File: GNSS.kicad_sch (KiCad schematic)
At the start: 0 parts

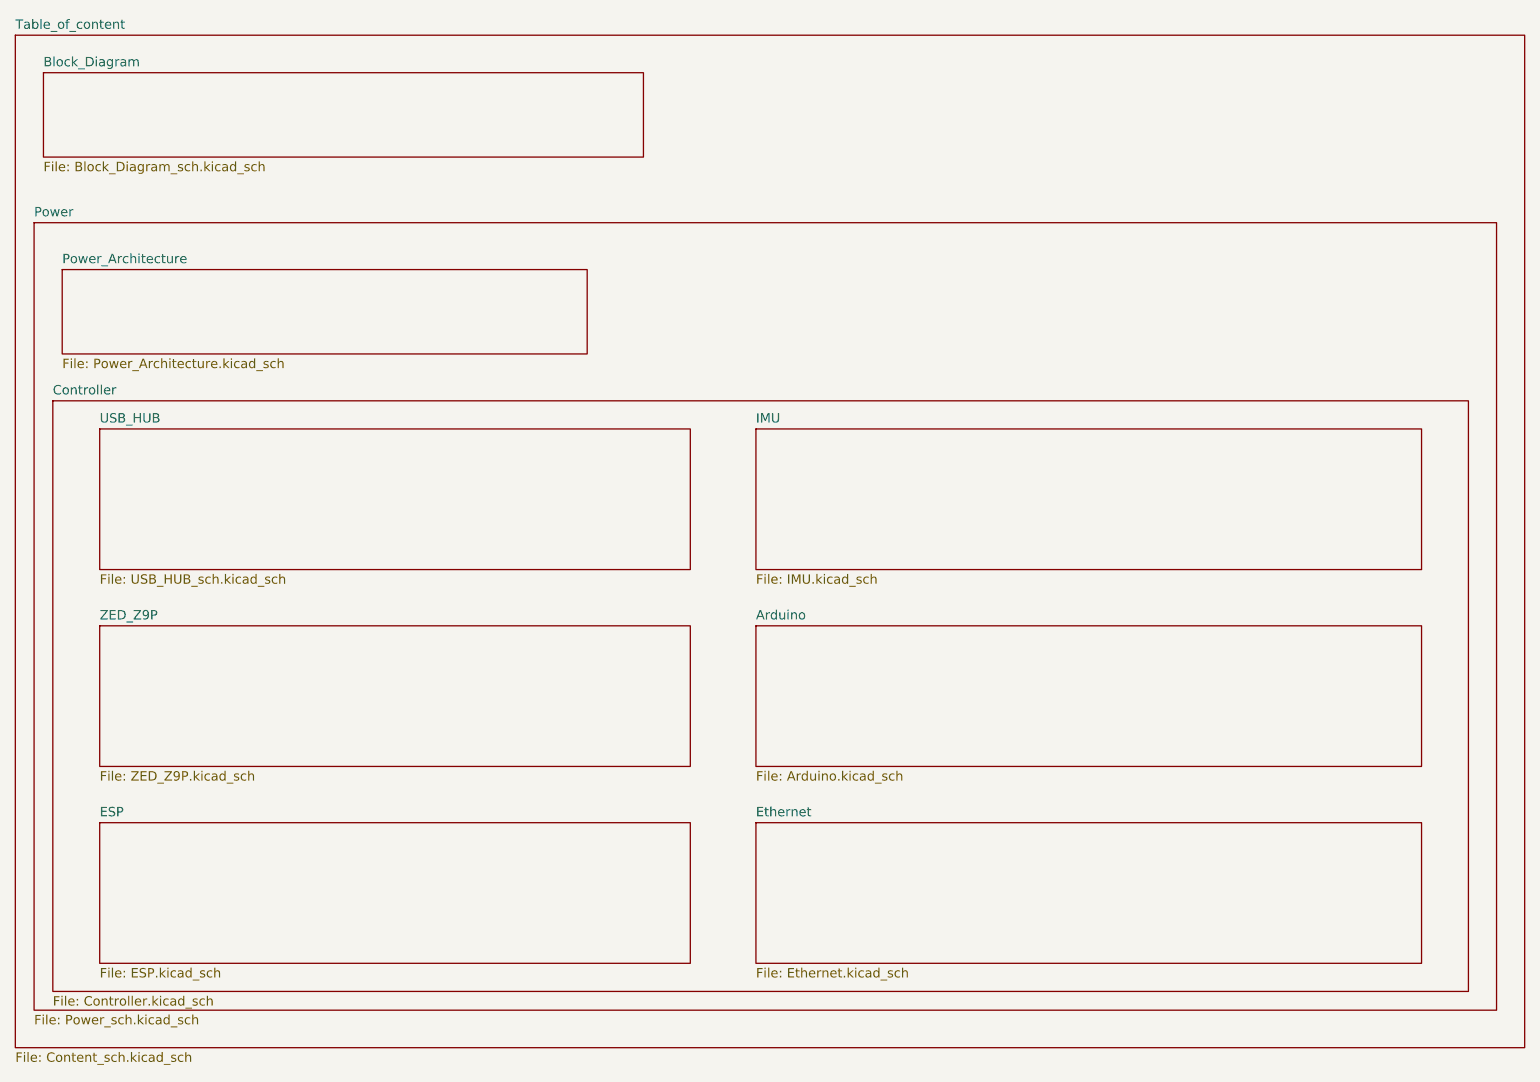
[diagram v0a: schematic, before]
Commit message: usb
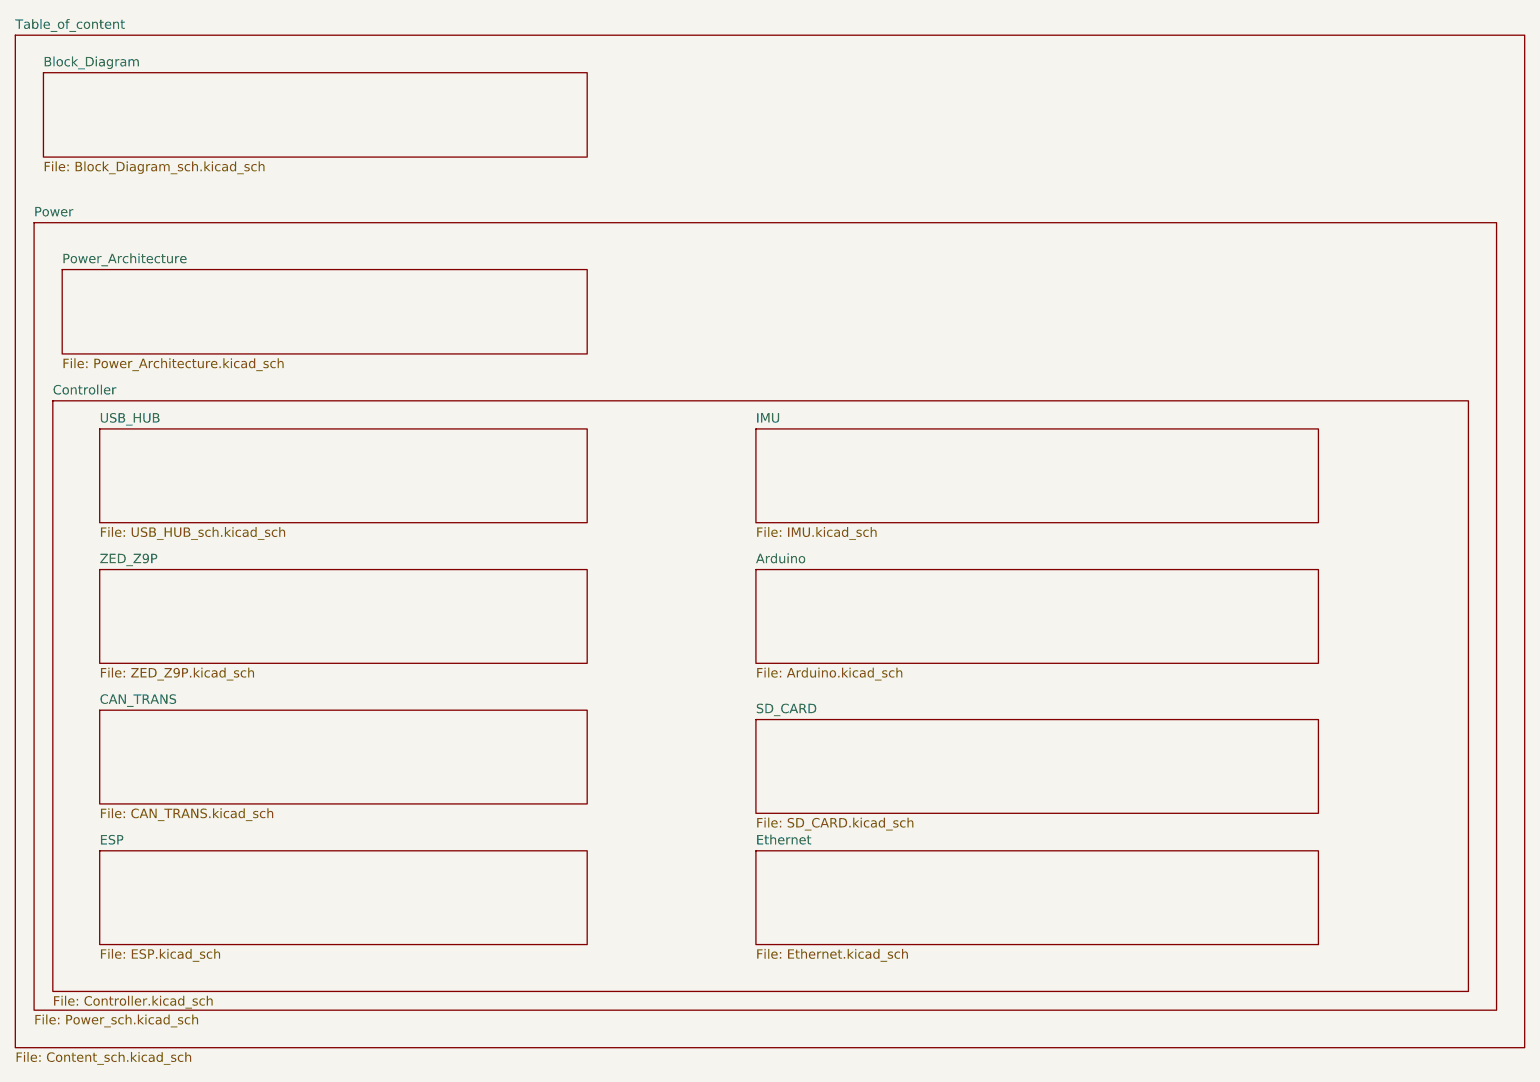
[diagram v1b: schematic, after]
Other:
- added sheet CAN_TRANS (CAN_TRANS.kicad_sch)
- added sheet SD_CARD (SD_CARD.kicad_sch)
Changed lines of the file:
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@@
 	(sheet
 		(at 137.16 74.93)
-		(size 90.17 19.05)
+		(size 76.2 12.7)
 		(fields_autoplaced yes)
 		(stroke
@@
 		)
 		(property "Sheetfile" "IMU.kicad_sch"
-			(at 137.16 94.5646 0)
+			(at 137.16 88.2146 0)
 			(effects
 				(font
@@
 	)
 	(sheet
-		(at 48.26 101.6)
-		(size 80.01 19.05)
+		(at 48.26 93.98)
+		(size 66.04 12.7)
 		(fields_autoplaced yes)
 		(stroke
@@
 		)
 		(property "Sheetname" "ZED_Z9P"
-			(at 48.26 100.8884 0)
+			(at 48.26 93.2684 0)
 			(effects
 				(font
@@
 		)
 		(property "Sheetfile" "ZED_Z9P.kicad_sch"
-			(at 48.26 121.2346 0)
+			(at 48.26 107.2646 0)
 			(effects
 				(font
@@
 	(sheet
 		(at 48.26 74.93)
-		(size 80.01 19.05)
+		(size 66.04 12.7)
 		(fields_autoplaced yes)
 		(stroke
@@
 		)
 		(property "Sheetfile" "USB_HUB_sch.kicad_sch"
-			(at 48.26 94.5646 0)
+			(at 48.26 88.2146 0)
 			(effects
 				(font
@@
 	(sheet
 		(at 40.64 26.67)
-		(size 81.28 11.43)
+		(size 73.66 11.43)
 		(fields_autoplaced yes)
 		(stroke
@@
 	)
 	(sheet
-		(at 137.16 128.27)
-		(size 90.17 19.05)
+		(at 137.16 132.08)
+		(size 76.2 12.7)
 		(fields_autoplaced yes)
 		(stroke
@@
 		)
 		(property "Sheetname" "Ethernet"
-			(at 137.16 127.5584 0)
+			(at 137.16 131.3684 0)
 			(effects
 				(font
@@
 		)
 		(property "Sheetfile" "Ethernet.kicad_sch"
-			(at 137.16 147.9046 0)
+			(at 137.16 145.3646 0)
 			(effects
 				(font
@@
 	)
 	(sheet
-		(at 137.16 101.6)
-		(size 90.17 19.05)
+		(at 137.16 93.98)
+		(size 76.2 12.7)
 		(fields_autoplaced yes)
 		(stroke
@@
 		)
 		(property "Sheetname" "Arduino"
-			(at 137.16 100.8884 0)
+			(at 137.16 93.2684 0)
 			(effects
 				(font
@@
 		)
 		(property "Sheetfile" "Arduino.kicad_sch"
-			(at 137.16 121.2346 0)
+			(at 137.16 107.2646 0)
 			(effects
 				(font
@@
 	)
 	(sheet
-		(at 48.26 128.27)
-		(size 80.01 19.05)
+		(at 137.16 114.3)
+		(size 76.2 12.7)
+		(fields_autoplaced yes)
+		(stroke
+			(width 0.1524)
+			(type solid)
+		)
+		(fill
+			(color 0 0 0 0.0000)
+		)
+		(property "Sheetname" "SD_CARD"
+			(at 137.16 113.5884 0)
+			(effects
+				(font
+					(size 1.27 1.27)
+				)
+				(justify left bottom)
+			)
+		)
+		(property "Sheetfile" "SD_CARD.kicad_sch"
+			(at 137.16 127.5846 0)
+			(effects
+				(font
+					(size 1.27 1.27)
+				)
+				(justify left top)
+			)
+		)
+		(instances
+			(project "GNSS"
+				(path "/a70dad34-b24c-4b58-b91c-f14576b5da7d"
+					(page "14")
+				)
+			)
+		)
+	)
+	(sheet
+		(at 48.26 132.08)
+		(size 66.04 12.7)
 		(fields_autoplaced yes)
 		(stroke
@@
 		)
 		(property "Sheetname" "ESP"
-			(at 48.26 127.5584 0)
+			(at 48.26 131.3684 0)
 			(effects
 				(font
@@
 		)
 		(property "Sheetfile" "ESP.kicad_sch"
-			(at 48.26 147.9046 0)
+			(at 48.26 145.3646 0)
 			(effects
 				(font
@@
 				)
 			)
+		)
+	)
+	(sheet
+		(at 48.26 113.03)
+		(size 66.04 12.7)
+		(fields_autoplaced yes)
+		(stroke
+			(width 0.1524)
+			(type solid)
+		)
+		(fill
+			(color 0 0 0 0.0000)
+		)
+		(property "Sheetname" "CAN_TRANS"
+			(at 48.26 112.3184 0)
+			(effects
+				(font
+					(size 1.27 1.27)
+				)
+				(justify left bottom)
+			)
+		)
+		(property "Sheetfile" "CAN_TRANS.kicad_sch"
+			(at 48.26 126.3146 0)
+			(effects
+				(font
+					(size 1.27 1.27)
+				)
+				(justify left top)
+			)
+		)
+		(instances
+			(project "GNSS"
+				(path "/a70dad34-b24c-4b58-b91c-f14576b5da7d"
+					(page "13")
+				)
+			)
